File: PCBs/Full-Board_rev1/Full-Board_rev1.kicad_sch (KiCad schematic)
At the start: 6 parts, among them U1 TPS630250RNCT

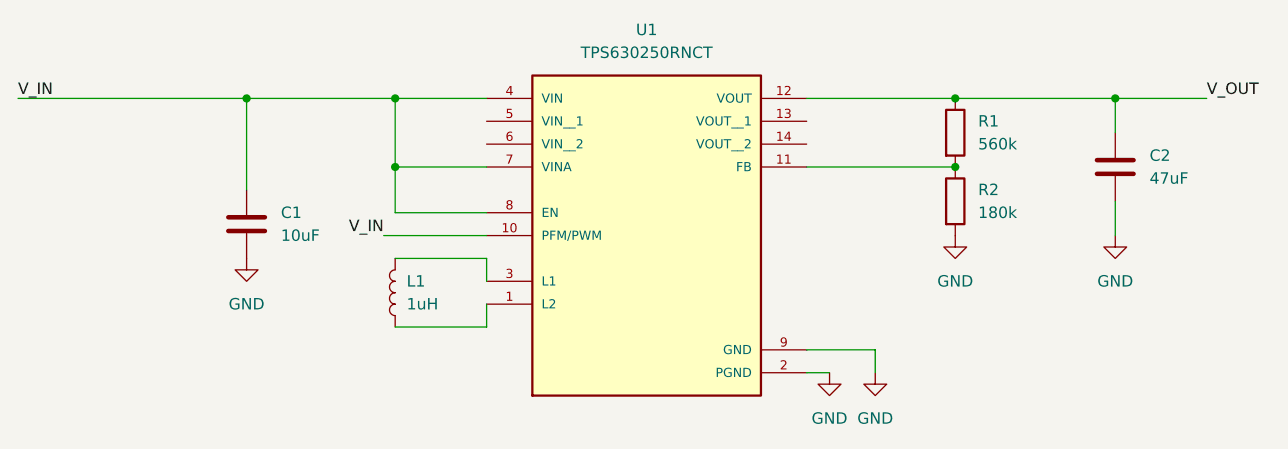
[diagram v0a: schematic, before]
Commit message: added modular design
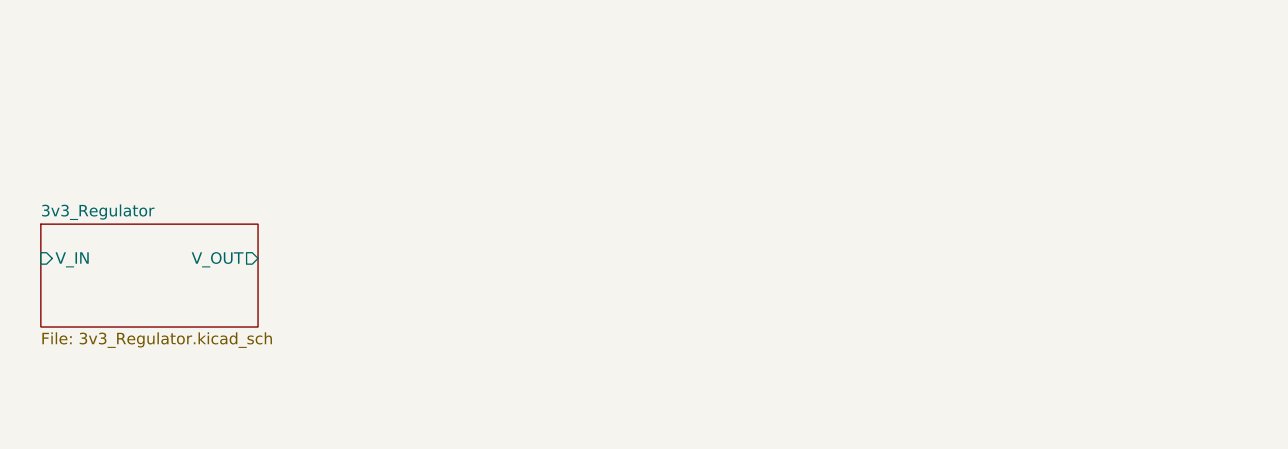
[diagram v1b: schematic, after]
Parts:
- removed C1: 10uF, symbol Device:C
- removed C2: 47uF, symbol Device:C
- removed L1: 1uH, symbol Device:L
- removed R1: 560k, symbol Device:R
- removed R2: 180k, symbol Device:R
- removed U1: TPS630250RNCT, TPS630250RNCT:VREG_TPS630250RNCT, symbol TPS630250RNCT:TPS630250RNCT
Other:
- added sheet 3v3_Regulator (3v3_Regulator.kicad_sch)
- title: (none) -> SwarmSolve PCB
